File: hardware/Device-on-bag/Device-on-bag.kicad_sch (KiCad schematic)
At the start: 3 parts, among them J1 Conn_01x12, J2 Conn_01x12, U2 mini_esp32

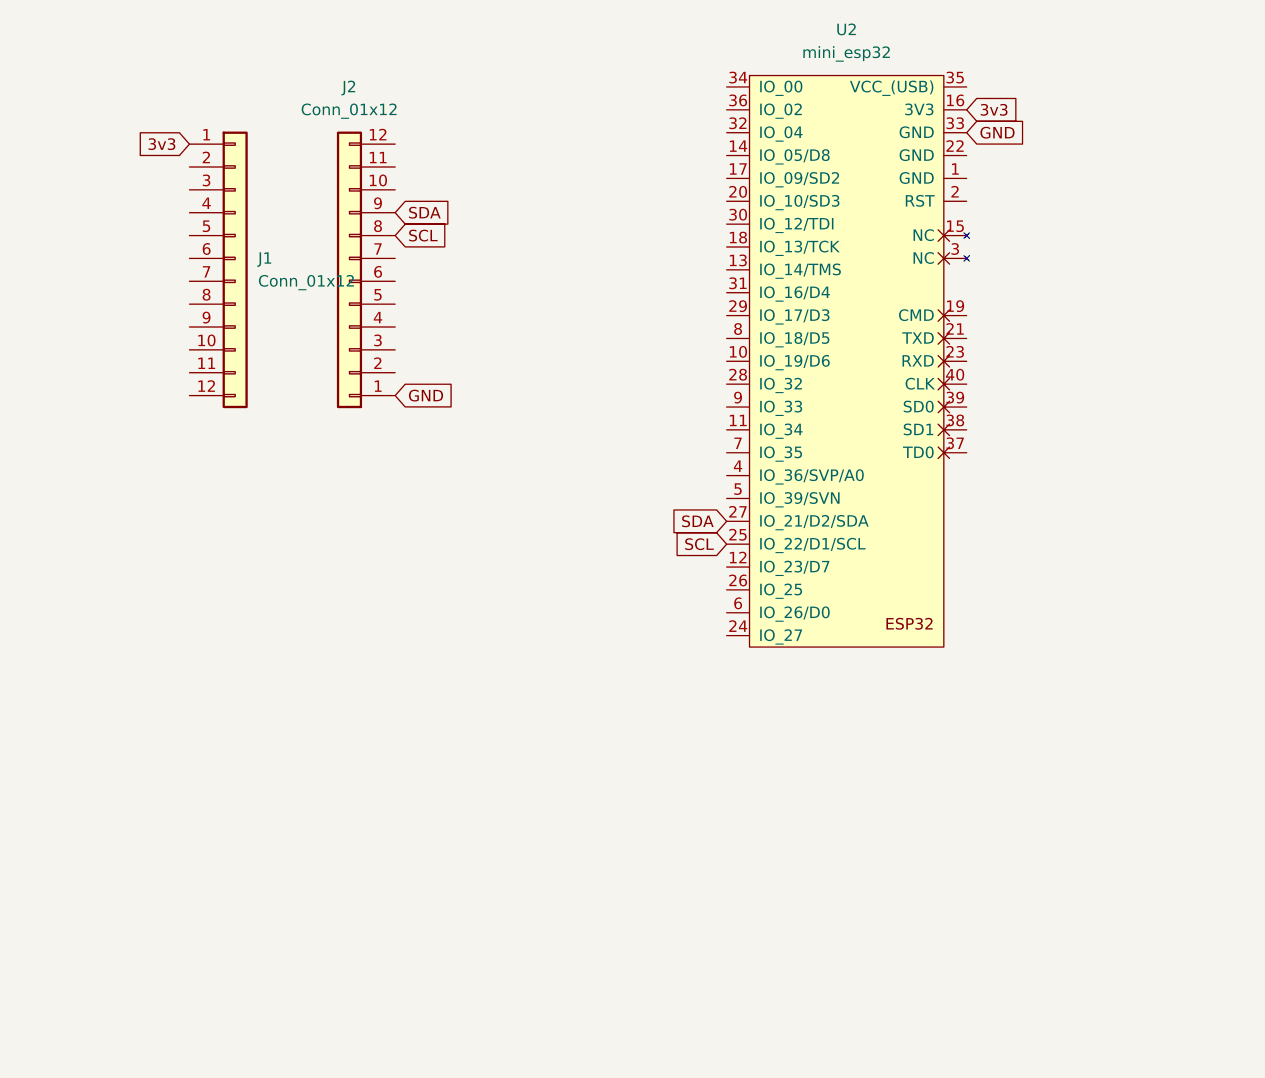
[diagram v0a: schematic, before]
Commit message: update
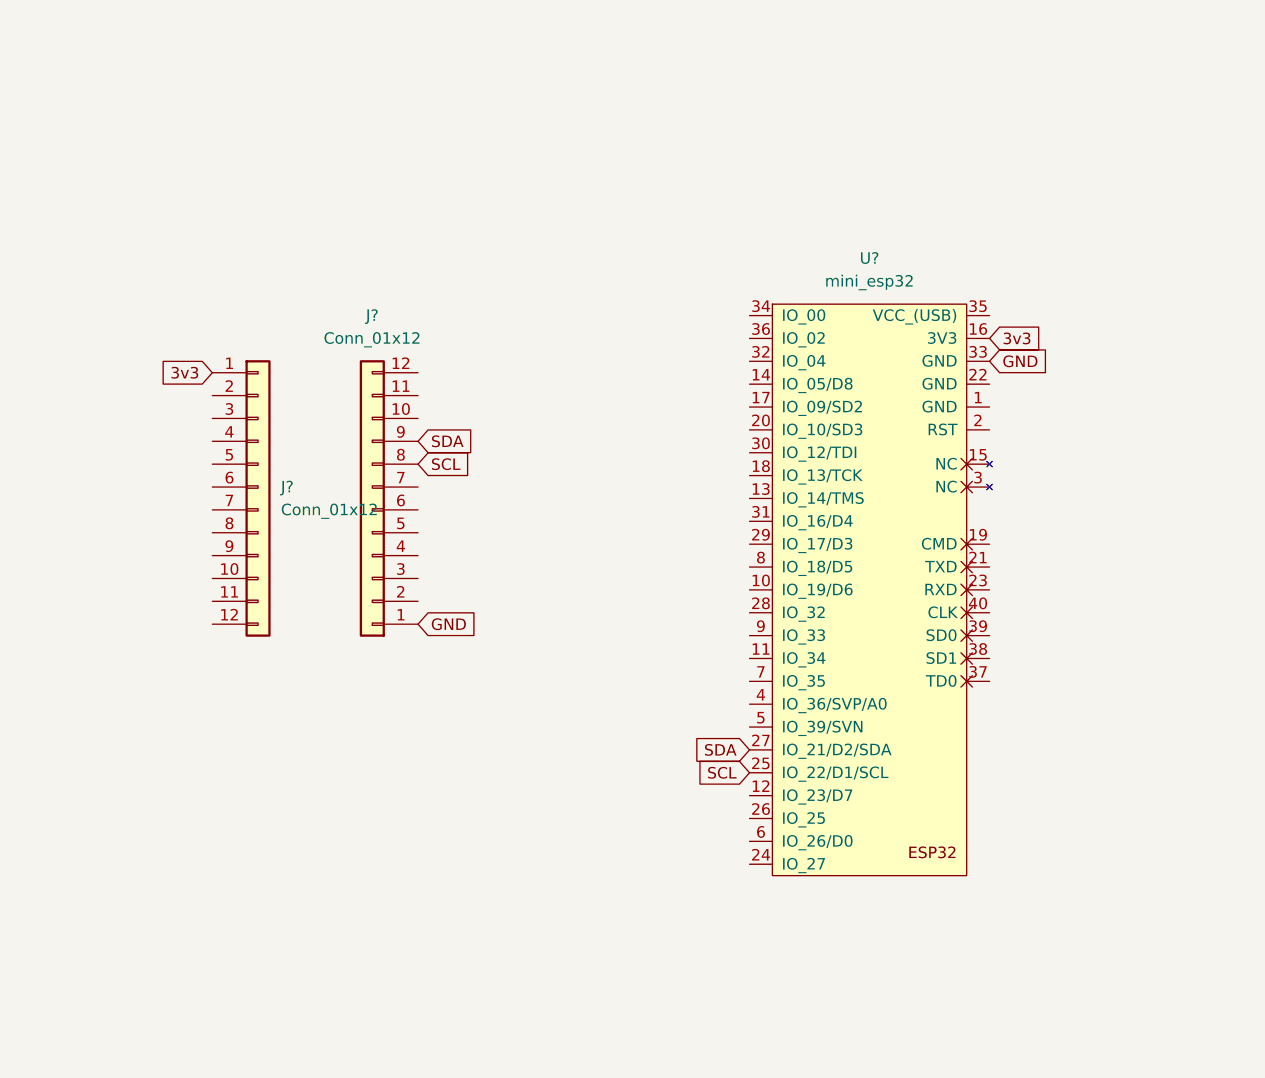
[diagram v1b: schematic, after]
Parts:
- removed J1, J2: Conn_01x12, Connector_PinSocket_2.54mm:PinSocket_1x11_P2.54mm_Vertical, symbol Connector_Generic:Conn_01x12
- removed U2: mini_esp32, ESP32_mini:ESP32_mini, symbol ESP32_mini:mini_esp32
- added J? (x2): Conn_01x12, Connector_PinSocket_2.54mm:PinSocket_1x11_P2.54mm_Vertical, symbol Connector_Generic:Conn_01x12
- added U?: mini_esp32, ESP32_mini:ESP32_mini, symbol ESP32_mini:mini_esp32
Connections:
- net 3v3: now also J?.1 (Pin_1), U?.16 (3V3)
- net GND: now also J?.1 (Pin_1), U?.33 (GND)
- net SCL: now also J?.8 (Pin_8), U?.25 (IO_22/D1/SCL)
- net SDA: now also J?.9 (Pin_9), U?.27 (IO_21/D2/SDA)
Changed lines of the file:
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@@
 (kicad_sch (version 20211123) (generator eeschema)
   (paper "A4")
-  (global_label "SCL" (shape input) (at 106.68 54.61 0) (fields_autoplaced)
+  (global_label "3v3" (shape input) (at 86.36 69.85 180) (fields_autoplaced)
+    (effects (font (size 1.27 1.27)) (justify right))
+    (property "Intersheet References" "${INTERSHEET_REFS}" (id 0) (at 80.5602 69.9294 0)
+      (effects (font (size 1.27 1.27)) (justify right) hide)
+    )
+  )
+  (global_label "SCL" (shape input) (at 146.05 114.3 180) (fields_autoplaced)
+    (effects (font (size 1.27 1.27)) (justify right))
+    (property "Intersheet References" "${INTERSHEET_REFS}" (id 0) (at 140.1293 114.3794 0)
+      (effects (font (size 1.27 1.27)) (justify right) hide)
+    )
+  )
+  (global_label "GND" (shape input) (at 172.72 68.58 0) (fields_autoplaced)
     (effects (font (size 1.27 1.27)) (justify left))
-    (property "Intersheet References" "${INTERSHEET_REFS}" (id 0) (at 112.6007 54.5306 0)
+    (property "Intersheet References" "${INTERSHEET_REFS}" (id 0) (at 179.0036 68.5006 0)
       (effects (font (size 1.27 1.27)) (justify left) hide)
     )
   )
-  (global_label "3v3" (shape input) (at 170.18 40.64 0) (fields_autoplaced)
+  (global_label "SCL" (shape input) (at 109.22 80.01 0) (fields_autoplaced)
     (effects (font (size 1.27 1.27)) (justify left))
-    (property "Intersheet References" "${INTERSHEET_REFS}" (id 0) (at 175.9798 40.5606 0)
+    (property "Intersheet References" "${INTERSHEET_REFS}" (id 0) (at 115.1407 79.9306 0)
       (effects (font (size 1.27 1.27)) (justify left) hide)
     )
   )
-  (global_label "GND" (shape input) (at 106.68 72.39 0) (fields_autoplaced)
+  (global_label "SDA" (shape input) (at 146.05 111.76 180) (fields_autoplaced)
+    (effects (font (size 1.27 1.27)) (justify right))
+    (property "Intersheet References" "${INTERSHEET_REFS}" (id 0) (at 140.0688 111.8394 0)
+      (effects (font (size 1.27 1.27)) (justify right) hide)
+    )
+  )
+  (global_label "GND" (shape input) (at 109.22 97.79 0) (fields_autoplaced)
     (effects (font (size 1.27 1.27)) (justify left))
-    (property "Intersheet References" "${INTERSHEET_REFS}" (id 0) (at 112.9636 72.3106 0)
+    (property "Intersheet References" "${INTERSHEET_REFS}" (id 0) (at 115.5036 97.7106 0)
       (effects (font (size 1.27 1.27)) (justify left) hide)
     )
   )
-  (global_label "SCL" (shape input) (at 143.51 88.9 180) (fields_autoplaced)
-    (effects (font (size 1.27 1.27)) (justify right))
-    (property "Intersheet References" "${INTERSHEET_REFS}" (id 0) (at 137.5893 88.9794 0)
-      (effects (font (size 1.27 1.27)) (justify right) hide)
-    )
-  )
-  (global_label "GND" (shape input) (at 170.18 43.18 0) (fields_autoplaced)
+  (global_label "3v3" (shape input) (at 172.72 66.04 0) (fields_autoplaced)
     (effects (font (size 1.27 1.27)) (justify left))
-    (property "Intersheet References" "${INTERSHEET_REFS}" (id 0) (at 176.4636 43.1006 0)
+    (property "Intersheet References" "${INTERSHEET_REFS}" (id 0) (at 178.5198 65.9606 0)
       (effects (font (size 1.27 1.27)) (justify left) hide)
     )
   )
-  (global_label "SDA" (shape input) (at 106.68 52.07 0) (fields_autoplaced)
+  (global_label "SDA" (shape input) (at 109.22 77.47 0) (fields_autoplaced)
     (effects (font (size 1.27 1.27)) (justify left))
-    (property "Intersheet References" "${INTERSHEET_REFS}" (id 0) (at 112.6612 51.9906 0)
+    (property "Intersheet References" "${INTERSHEET_REFS}" (id 0) (at 115.2012 77.3906 0)
       (effects (font (size 1.27 1.27)) (justify left) hide)
     )
   )
-  (global_label "3v3" (shape input) (at 83.82 44.45 180) (fields_autoplaced)
-    (effects (font (size 1.27 1.27)) (justify right))
-    (property "Intersheet References" "${INTERSHEET_REFS}" (id 0) (at 78.0202 44.5294 0)
-      (effects (font (size 1.27 1.27)) (justify right) hide)
-    )
-  )
-  (global_label "SDA" (shape input) (at 143.51 86.36 180) (fields_autoplaced)
-    (effects (font (size 1.27 1.27)) (justify right))
-    (property "Intersheet References" "${INTERSHEET_REFS}" (id 0) (at 137.5288 86.4394 0)
-      (effects (font (size 1.27 1.27)) (justify right) hide)
-    )
-  )
-  (symbol (lib_id "Connector_Generic:Conn_01x12") (at 88.9 57.15 0) (unit 1)
+  (symbol (lib_id "ESP32_mini:mini_esp32") (at 158.75 60.96 0) (unit 1)
     (in_bom yes) (on_board yes) (fields_autoplaced)
-    (property "Reference" "J1" (id 0) (at 91.44 57.1499 0)
-      (effects (font (size 1.27 1.27)) (justify left))
-    )
-    (property "Value" "Conn_01x12" (id 1) (at 91.44 59.6899 0)
-      (effects (font (size 1.27 1.27)) (justify left))
-    )
-    (property "Footprint" "Connector_PinSocket_2.54mm:PinSocket_1x11_P2.54mm_Vertical" (id 2) (at 88.9 57.15 0)
+    (property "Reference" "U?" (id 0) (at 159.385 57.15 0))
+    (property "Value" "mini_esp32" (id 1) (at 159.385 59.69 0))
+    (property "Footprint" "ESP32_mini:ESP32_mini" (id 2) (at 162.56 58.42 0)
       (effects (font (size 1.27 1.27)) hide)
     )
-    (property "Datasheet" "~" (id 3) (at 88.9 57.15 0)
-      (effects (font (size 1.27 1.27)) hide)
-    )
-    (pin "1")
-    (pin "10")
-    (pin "11")
-    (pin "12")
-    (pin "2")
-    (pin "3")
-    (pin "4")
-    (pin "5")
-    (pin "6")
-    (pin "7")
-    (pin "8")
-    (pin "9")
-  )
-  (symbol (lib_id "ESP32_mini:mini_esp32") (at 156.21 35.56 0) (unit 1)
-    (in_bom yes) (on_board yes) (fields_autoplaced)
-    (property "Reference" "U2" (id 0) (at 156.845 31.75 0))
-    (property "Value" "mini_esp32" (id 1) (at 156.845 34.29 0))
-    (property "Footprint" "ESP32_mini:ESP32_mini" (id 2) (at 160.02 33.02 0)
-      (effects (font (size 1.27 1.27)) hide)
-    )
-    (property "Datasheet" "" (id 3) (at 160.02 33.02 0)
+    (property "Datasheet" "" (id 3) (at 162.56 58.42 0)
       (effects (font (size 1.27 1.27)) hide)
     )
@@
     (pin "9")
   )
-  (symbol (lib_id "Connector_Generic:Conn_01x12") (at 101.6 59.69 180) (unit 1)
+  (symbol (lib_id "Connector_Generic:Conn_01x12") (at 91.44 82.55 0) (unit 1)
     (in_bom yes) (on_board yes) (fields_autoplaced)
-    (property "Reference" "J2" (id 0) (at 101.6 38.1 0))
-    (property "Value" "Conn_01x12" (id 1) (at 101.6 40.64 0))
-    (property "Footprint" "Connector_PinSocket_2.54mm:PinSocket_1x11_P2.54mm_Vertical" (id 2) (at 101.6 59.69 0)
+    (property "Reference" "J?" (id 0) (at 93.98 82.5499 0)
+      (effects (font (size 1.27 1.27)) (justify left))
+    )
+    (property "Value" "Conn_01x12" (id 1) (at 93.98 85.0899 0)
+      (effects (font (size 1.27 1.27)) (justify left))
+    )
+    (property "Footprint" "Connector_PinSocket_2.54mm:PinSocket_1x11_P2.54mm_Vertical" (id 2) (at 91.44 82.55 0)
       (effects (font (size 1.27 1.27)) hide)
     )
-    (property "Datasheet" "~" (id 3) (at 101.6 59.69 0)
+    (property "Datasheet" "~" (id 3) (at 91.44 82.55 0)
+      (effects (font (size 1.27 1.27)) hide)
+    )
+    (pin "1")
+    (pin "10")
+    (pin "11")
+    (pin "12")
+    (pin "2")
+    (pin "3")
+    (pin "4")
+    (pin "5")
+    (pin "6")
+    (pin "7")
+    (pin "8")
+    (pin "9")
+  )
+  (symbol (lib_id "Connector_Generic:Conn_01x12") (at 104.14 85.09 180) (unit 1)
+    (in_bom yes) (on_board yes) (fields_autoplaced)
+    (property "Reference" "J?" (id 0) (at 104.14 63.5 0))
+    (property "Value" "Conn_01x12" (id 1) (at 104.14 66.04 0))
+    (property "Footprint" "Connector_PinSocket_2.54mm:PinSocket_1x11_P2.54mm_Vertical" (id 2) (at 104.14 85.09 0)
+      (effects (font (size 1.27 1.27)) hide)
+    )
+    (property "Datasheet" "~" (id 3) (at 104.14 85.09 0)
       (effects (font (size 1.27 1.27)) hide)
     )
@@
   )
   (symbol_instances
-    (path "/564d691c-9f25-47d5-a421-d002b9a03357"
-      (reference "J1") (unit 1) (value "Conn_01x12") (footprint "Connector_PinSocket_2.54mm:PinSocket_1x11_P2.54mm_Vertical")
+    (path "/b65a8ad3-ec23-4ae3-b007-02d5070d82ec"
+      (reference "J?") (unit 1) (value "Conn_01x12") (footprint "Connector_PinSocket_2.54mm:PinSocket_1x11_P2.54mm_Vertical")
     )
-    (path "/95489415-dcfc-4ecb-91af-091a7dad7566"
-      (reference "J2") (unit 1) (value "Conn_01x12") (footprint "Connector_PinSocket_2.54mm:PinSocket_1x11_P2.54mm_Vertical")
+    (path "/def40bea-bd6a-4bd4-85d6-38a0bc393684"
+      (reference "J?") (unit 1) (value "Conn_01x12") (footprint "Connector_PinSocket_2.54mm:PinSocket_1x11_P2.54mm_Vertical")
     )
-    (path "/776caef5-77e8-479d-9002-efa59d947083"
-      (reference "U2") (unit 1) (value "mini_esp32") (footprint "ESP32_mini:ESP32_mini")
+    (path "/1f881f44-1f04-46f4-a465-f1747e7275b2"
+      (reference "U?") (unit 1) (value "mini_esp32") (footprint "ESP32_mini:ESP32_mini")
     )
   )
